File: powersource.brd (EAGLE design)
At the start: 95.1 x 72.2 mm, 11 parts

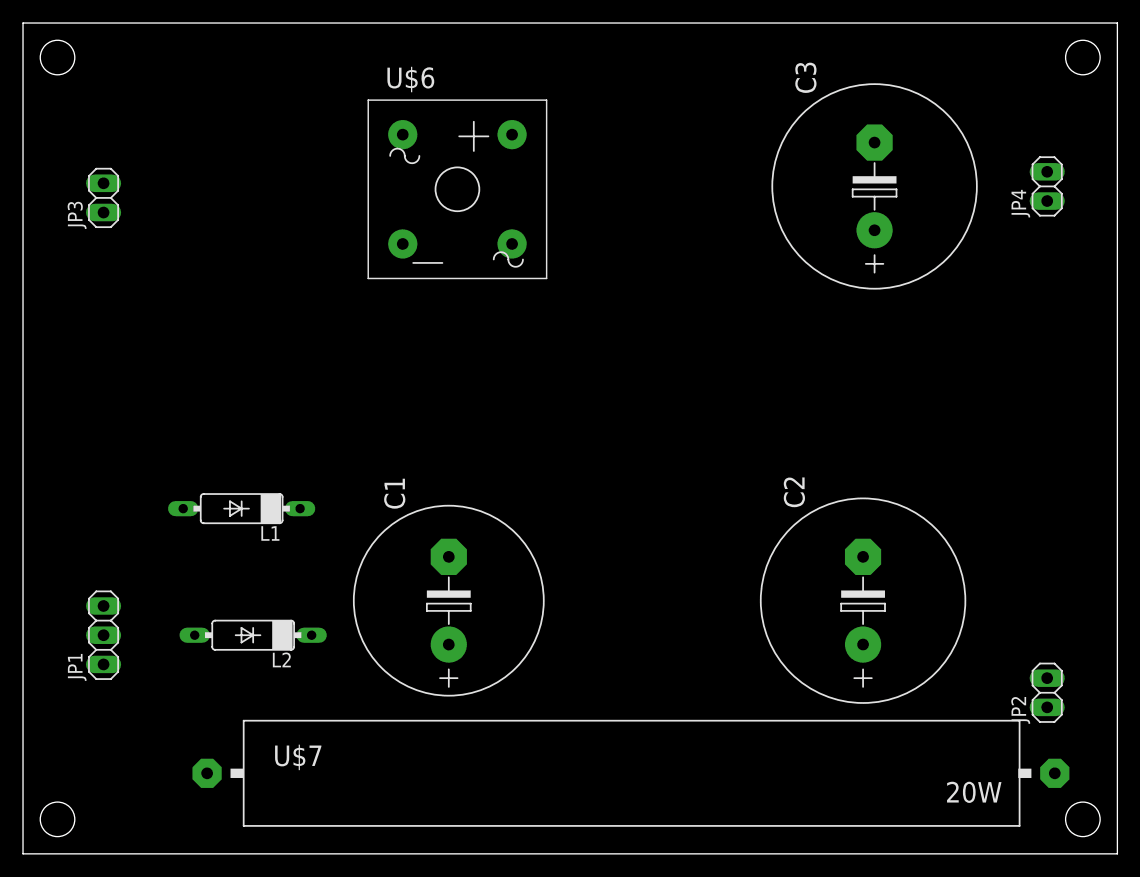
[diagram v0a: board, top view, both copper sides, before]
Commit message: [fix]超超微調整
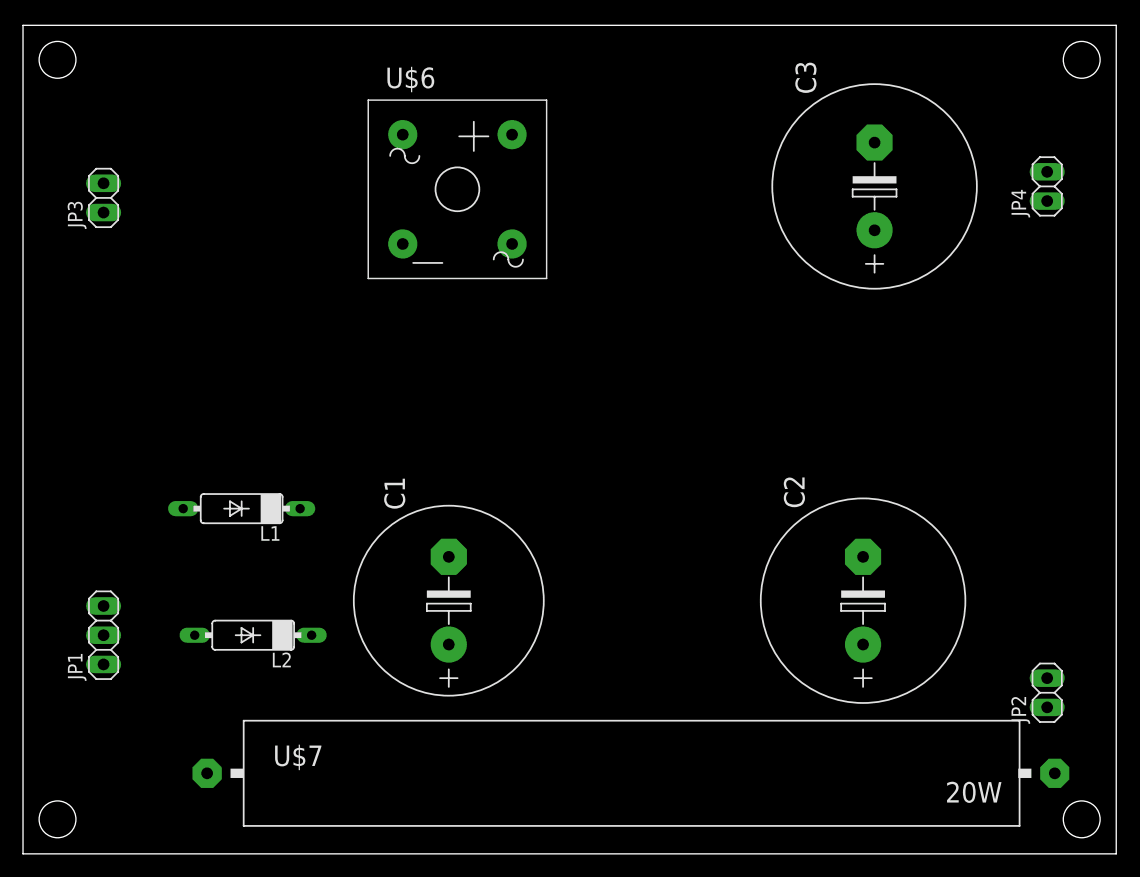
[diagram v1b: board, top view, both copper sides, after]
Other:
- board size 95.1 x 72.2 mm -> 95 x 72 mm
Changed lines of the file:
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@@
 </layers>
 <board>
-<fusionsync huburn="a.cGVyc29uYWw6dWUyZDlmMDVj" projecturn="a.cGVyc29uYWw6dWUyZDlmMDVjIzIwMTgxMjMwMTY3NjU5OTU2" f3durn="urn:adsk.wipprod:dm.lineage:1p4ZNr76QF6s9D04_b7MiQ" pcbguid="6f970ecf-14a9-49a9-a88c-6c1ebdaac8da" lastpulledtime="" lastsyncedchangeguid="05b6d938-cdf6-f8e0-c3d8-3ea724515d47"/>
+<fusionsync huburn="a.cGVyc29uYWw6dWUyZDlmMDVj" projecturn="a.cGVyc29uYWw6dWUyZDlmMDVjIzIwMTgxMjMwMTY3NjU5OTU2" f3durn="urn:adsk.wipprod:dm.lineage:1p4ZNr76QF6s9D04_b7MiQ" pcbguid="6f970ecf-14a9-49a9-a88c-6c1ebdaac8da" lastpulledtime="" lastsyncedchangeguid="dffcab59-db55-236d-5594-2eaaafb1d0d9"/>
 <plain>
-<wire x1="0" y1="0" x2="95.1" y2="0" width="0" layer="20"/>
-<wire x1="95.1" y1="0" x2="95.1" y2="72.2" width="0" layer="20"/>
-<wire x1="95.1" y1="72.2" x2="0" y2="72.2" width="0" layer="20"/>
-<wire x1="0" y1="72.2" x2="0" y2="0" width="0" layer="20"/>
-<hole x="3" y="3" drill="3"/>
-<hole x="92.1" y="3" drill="3"/>
-<hole x="3" y="69.2" drill="3"/>
-<hole x="92.1" y="69.2" drill="3"/>
+<wire x1="0" y1="0" x2="95" y2="0" width="0" layer="20"/>
+<wire x1="95" y1="0" x2="95" y2="72" width="0" layer="20"/>
+<wire x1="95" y1="72" x2="0" y2="72" width="0" layer="20"/>
+<wire x1="0" y1="72" x2="0" y2="0" width="0" layer="20"/>
+<hole x="3" y="3" drill="3.2"/>
+<hole x="92" y="3" drill="3.2"/>
+<hole x="3" y="69" drill="3.2"/>
+<hole x="92" y="69" drill="3.2"/>
 </plain>
 <attributes>
@@
 <attribute name="VALUE" x="92.175" y="55.46" size="1.27" layer="27" rot="R90"/>
 </element>
-<element name="C1" library="VacuumTube" library_urn="urn:adsk.eagle:library:8044196" package="E7,5-16" package3d_urn="urn:adsk.eagle:package:8399792/1" value="E7.5-16" x="37" y="22" smashed="yes" rot="R90">
+<element name="C1" library="VacuumTube" library_urn="urn:adsk.eagle:library:8044196" package="E7,5-16" package3d_urn="urn:adsk.eagle:package:8399792/3" value="E7.5-16" x="37" y="22" smashed="yes" rot="R90">
 <attribute name="NAME" x="33.19" y="29.874" size="1.778" layer="25" ratio="10" rot="R90"/>
 <attribute name="VALUE" x="41.2926" y="16.92" size="1.778" layer="27" ratio="10" rot="R90"/>
 </element>
-<element name="C2" library="VacuumTube" library_urn="urn:adsk.eagle:library:8044196" package="E7,5-18" package3d_urn="urn:adsk.eagle:package:8399793/1" value="E7.5-18" x="73" y="22" smashed="yes" rot="R90">
+<element name="C2" library="VacuumTube" library_urn="urn:adsk.eagle:library:8044196" package="E7,5-18" package3d_urn="urn:adsk.eagle:package:8399793/3" value="E7.5-18" x="73" y="22" smashed="yes" rot="R90">
 <attribute name="NAME" x="67.92" y="30.001" size="1.778" layer="25" ratio="10" rot="R90"/>
 <attribute name="VALUE" x="77.2926" y="16.92" size="1.778" layer="27" ratio="10" rot="R90"/>
 </element>
-<element name="C3" library="VacuumTube" library_urn="urn:adsk.eagle:library:8044196" package="E7,5-18" package3d_urn="urn:adsk.eagle:package:8399793/1" value="E7.5-18" x="74" y="58" smashed="yes" rot="R90">
+<element name="C3" library="VacuumTube" library_urn="urn:adsk.eagle:library:8044196" package="E7,5-18" package3d_urn="urn:adsk.eagle:package:8399793/3" value="E7.5-18" x="74" y="58" smashed="yes" rot="R90">
 <attribute name="NAME" x="68.92" y="66.001" size="1.778" layer="25" ratio="10" rot="R90"/>
 <attribute name="VALUE" x="78.2926" y="52.92" size="1.778" layer="27" ratio="10" rot="R90"/>
@@
 <attribute name="VALUE" x="34.555" y="52.92" size="1.778" layer="27" ratio="10"/>
 </element>
-<element name="U$7" library="VacuumTube" library_urn="urn:adsk.eagle:library:8044196" package="RESISTOR" package3d_urn="urn:adsk.eagle:package:8399790/1" value="RESISTOR" x="16" y="7" smashed="yes">
+<element name="U$7" library="VacuumTube" library_urn="urn:adsk.eagle:library:8044196" package="RESISTOR" package3d_urn="urn:adsk.eagle:package:8399790/2" value="RESISTOR" x="16" y="7" smashed="yes">
 <attribute name="NAME" x="21.715" y="7.635" size="1.778" layer="25" ratio="10"/>
 <attribute name="VALUE" x="21.715" y="4.46" size="1.778" layer="27" ratio="10"/>
